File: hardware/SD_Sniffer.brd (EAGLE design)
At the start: 73.7 x 34.8 mm, 10 parts, among them U1 SD_CARD_SOCKET, U2 SD_MMC_CARDSD_PCB

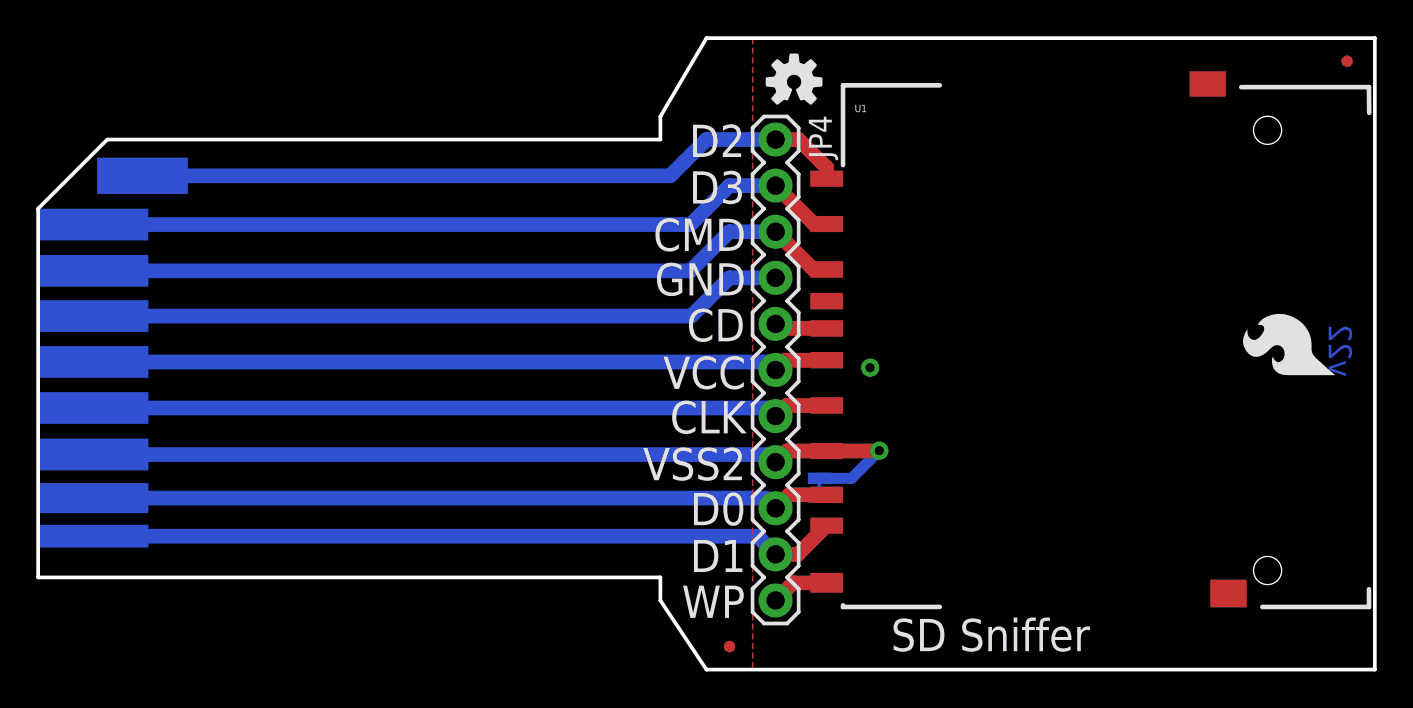
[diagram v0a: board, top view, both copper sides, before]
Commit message: Fixed eagle sync
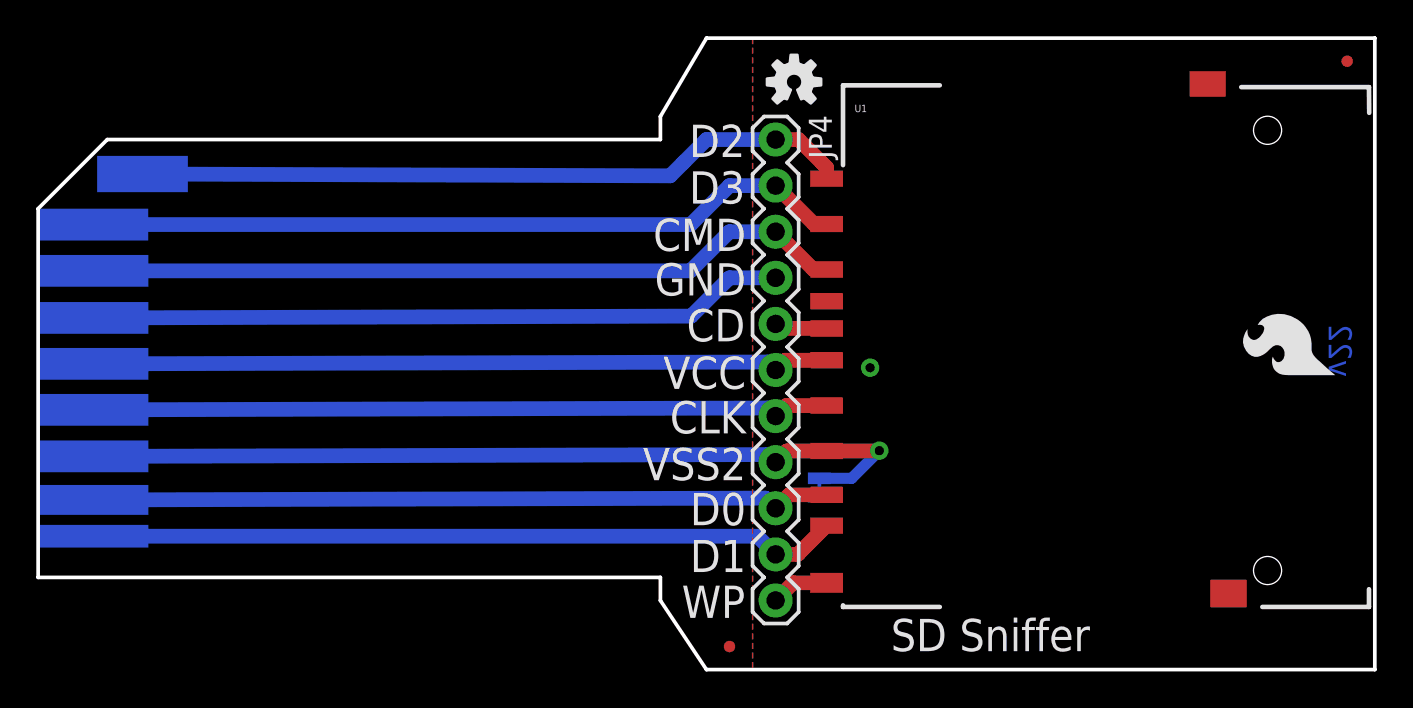
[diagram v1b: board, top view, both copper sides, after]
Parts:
- U2: device SparkFun:SD-MMC-CARD@1 -> SparkFun-Boards:SD-MMC-CARD
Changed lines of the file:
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@@
 <layer number="27" name="tValues" color="7" fill="1" visible="no" active="yes"/>
 <layer number="28" name="bValues" color="7" fill="1" visible="no" active="yes"/>
-<layer number="29" name="tStop" color="7" fill="3" visible="yes" active="yes"/>
+<layer number="29" name="tStop" color="7" fill="3" visible="no" active="yes"/>
 <layer number="30" name="bStop" color="7" fill="6" visible="no" active="yes"/>
 <layer number="31" name="tCream" color="7" fill="4" visible="no" active="yes"/>
@@
 </autorouter>
 <elements>
-<element name="U2" library="SparkFun" package="SD-MMC-CARD@1" value="SD_MMC_CARDSD_PCB" x="17.78" y="16.51" smashed="yes" rot="MR270">
+<element name="U2" library="SparkFun-Boards" package="SD-MMC-CARD" value="SD_MMC_CARDSD_PCB" x="17.78" y="16.51" smashed="yes" rot="MR270">
 <attribute name="NAME" x="-1.27" y="21.59" size="0.4064" layer="26" rot="MR90"/>
 <attribute name="VALUE" x="-1.27" y="10.16" size="0.4064" layer="28" rot="MR90"/>
@@
 <wire x1="40.64" y1="27.94" x2="36.83" y2="27.94" width="0.8128" layer="16"/>
 <wire x1="36.83" y1="27.94" x2="35.56" y2="26.67" width="0.8128" layer="16"/>
-<wire x1="5.75" y1="25.94" x2="34.83" y2="25.94" width="0.8128" layer="16"/>
+<wire x1="5.75" y1="26.04" x2="34.83" y2="25.94" width="0.8128" layer="16"/>
 <wire x1="34.83" y1="25.94" x2="35.56" y2="26.67" width="0.8128" layer="16"/>
 </signal>
@@
 <via x="45.847" y="15.367" extent="1-16" drill="0.508"/>
 <contactref element="JP4" pad="4"/>
-<wire x1="3.077" y1="18.21" x2="35.99" y2="18.21" width="0.8128" layer="16"/>
+<wire x1="3.077" y1="18.11" x2="35.99" y2="18.21" width="0.8128" layer="16"/>
 <wire x1="35.99" y1="18.21" x2="38.1" y2="20.32" width="0.8128" layer="16"/>
 <wire x1="38.1" y1="20.32" x2="40.64" y2="20.32" width="0.8128" layer="16"/>
@@
 <contactref element="U1" pad="5"/>
 <contactref element="JP4" pad="7"/>
-<wire x1="3.077" y1="13.145" x2="40.195" y2="13.145" width="0.8128" layer="16"/>
+<wire x1="3.077" y1="13.045" x2="40.195" y2="13.145" width="0.8128" layer="16"/>
 <wire x1="40.195" y1="13.145" x2="40.64" y2="12.7" width="0.8128" layer="16"/>
 <wire x1="43.45" y1="13.28" x2="41.22" y2="13.28" width="0.8128" layer="1"/>
@@
 <contactref element="U1" pad="7"/>
 <contactref element="JP4" pad="9"/>
-<wire x1="3.077" y1="8.18" x2="40.08" y2="8.18" width="0.8128" layer="16"/>
+<wire x1="3.077" y1="8.08" x2="40.08" y2="8.18" width="0.8128" layer="16"/>
 <wire x1="40.08" y1="8.18" x2="40.64" y2="7.62" width="0.8128" layer="16"/>
 <wire x1="43.45" y1="8.36" x2="41.38" y2="8.36" width="0.8128" layer="1"/>
@@
 <contactref element="U2" pad="4"/>
 <contactref element="JP4" pad="6"/>
-<wire x1="3.077" y1="15.68" x2="40.2" y2="15.68" width="0.8128" layer="16"/>
+<wire x1="3.077" y1="15.58" x2="40.2" y2="15.68" width="0.8128" layer="16"/>
 <wire x1="40.2" y1="15.68" x2="40.64" y2="15.24" width="0.8128" layer="16"/>
 <wire x1="43.45" y1="15.78" x2="41.18" y2="15.78" width="0.8128" layer="1"/>
@@
 <contactref element="SJ1" pad="2"/>
 <contactref element="JP4" pad="8"/>
-<wire x1="3.077" y1="10.58" x2="40.22" y2="10.58" width="0.8128" layer="16"/>
+<wire x1="3.077" y1="10.48" x2="40.22" y2="10.58" width="0.8128" layer="16"/>
 <wire x1="40.22" y1="10.58" x2="40.64" y2="10.16" width="0.8128" layer="16"/>
 <wire x1="43.45" y1="10.78" x2="41.26" y2="10.78" width="0.8128" layer="1"/>
